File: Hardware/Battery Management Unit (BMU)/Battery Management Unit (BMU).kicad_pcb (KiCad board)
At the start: 4 copper layers, 105 x 65.5 mm, 93 parts, among them IC1 STM32C092RCT6, J1 HIGH SIDE, J10 SHUNT, J11 ALERT, J12 CAN, J13 Conn_ST_STDC14, J2 LOW SIDE, J3 POWER, J4 GPIO, J5 GND, J6 5V, J7 3V3, J8 FAULT, J9 I2C, Q1 DMP3099L, SW1 Power Switch, SW2 RESET Switch, T1 CEP99-102, T2 CEP99-102, U1 OKI-78SR-5_1.5-W36-C, U2 TLV75533PDBV, U3 PESD5V0L2BT, U4 BQ79600PWRQ1, U5 PESD5V0L2BT, U6 MCP2562FDT-H_SN

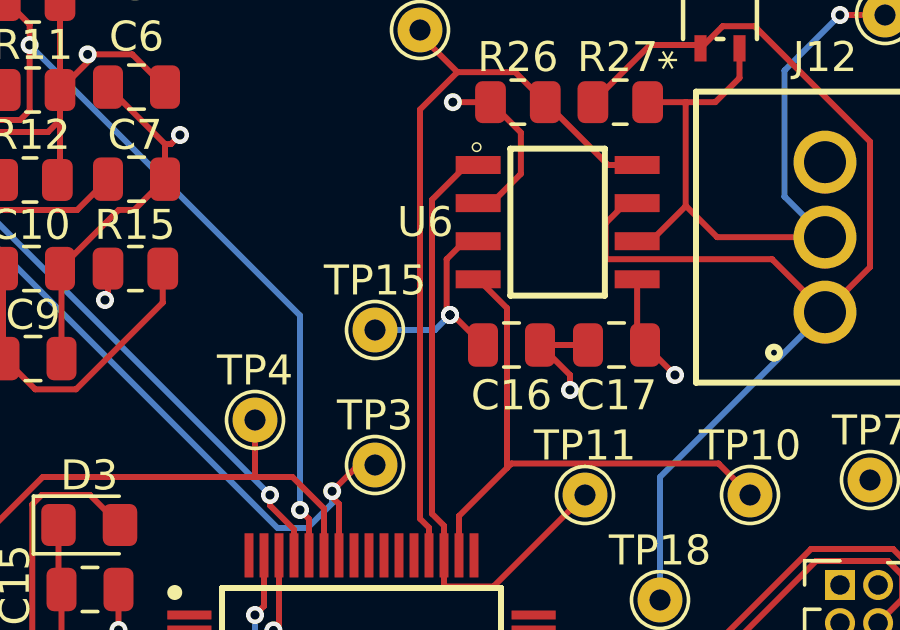
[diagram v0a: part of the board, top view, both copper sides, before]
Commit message: update layout
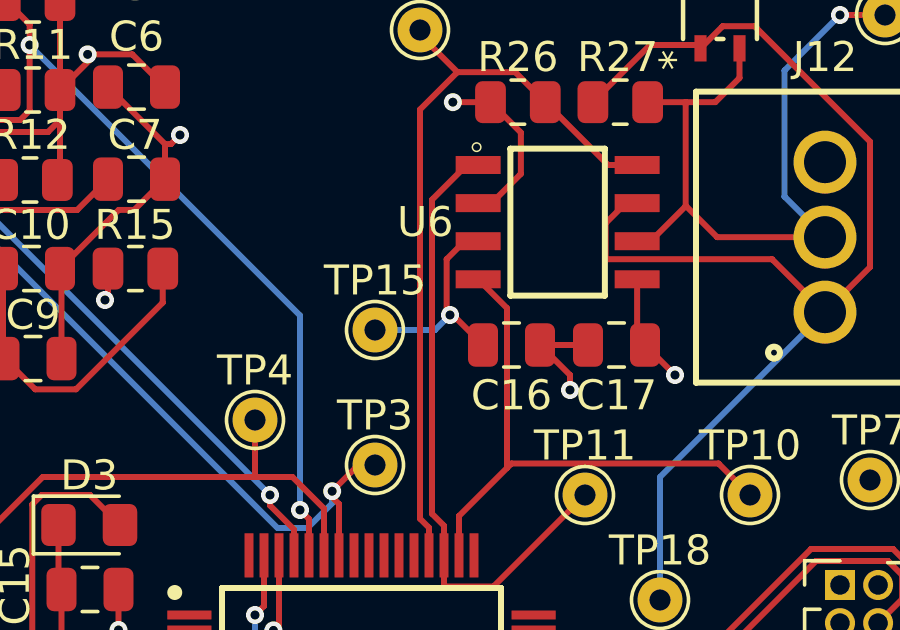
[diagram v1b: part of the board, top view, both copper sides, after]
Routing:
- net +5V: vias 5 -> 4
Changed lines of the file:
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@@
-	)
-	(via
-		(at 171.5 102.5)
-		(size 0.6)
-		(drill 0.3)
-		(layers "F.Cu" "B.Cu")
-		(net "+5V")
 	)
 	(via
